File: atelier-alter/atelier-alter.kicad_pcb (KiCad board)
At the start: 2 copper layers, 81.3 x 80 mm, 59 parts, among them SW1 SW_DPST, SW2 SW_DPST, SW3 SW_DPST, SW4 RESET, U1 ATmega32U4-A, U2 PRTR5V0U2X, Y1 16Mhz

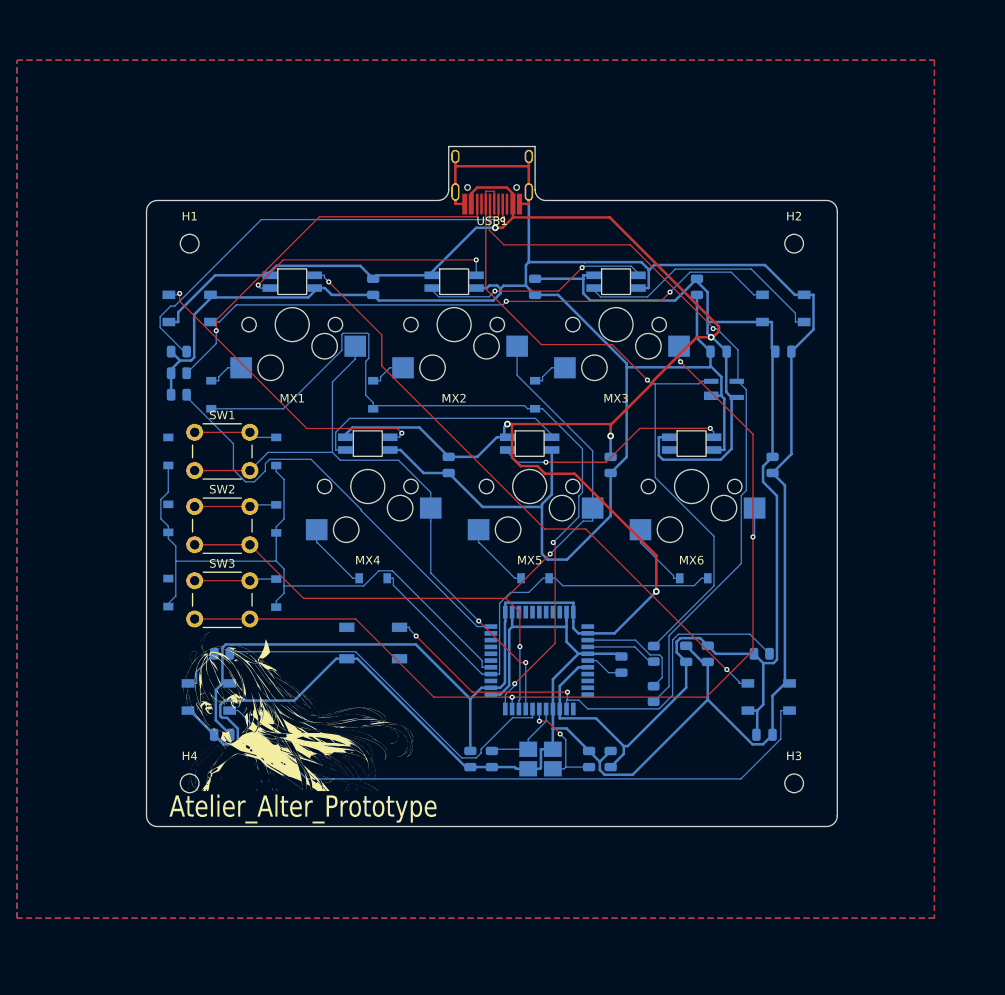
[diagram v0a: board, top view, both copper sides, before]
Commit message: minor updates here and there
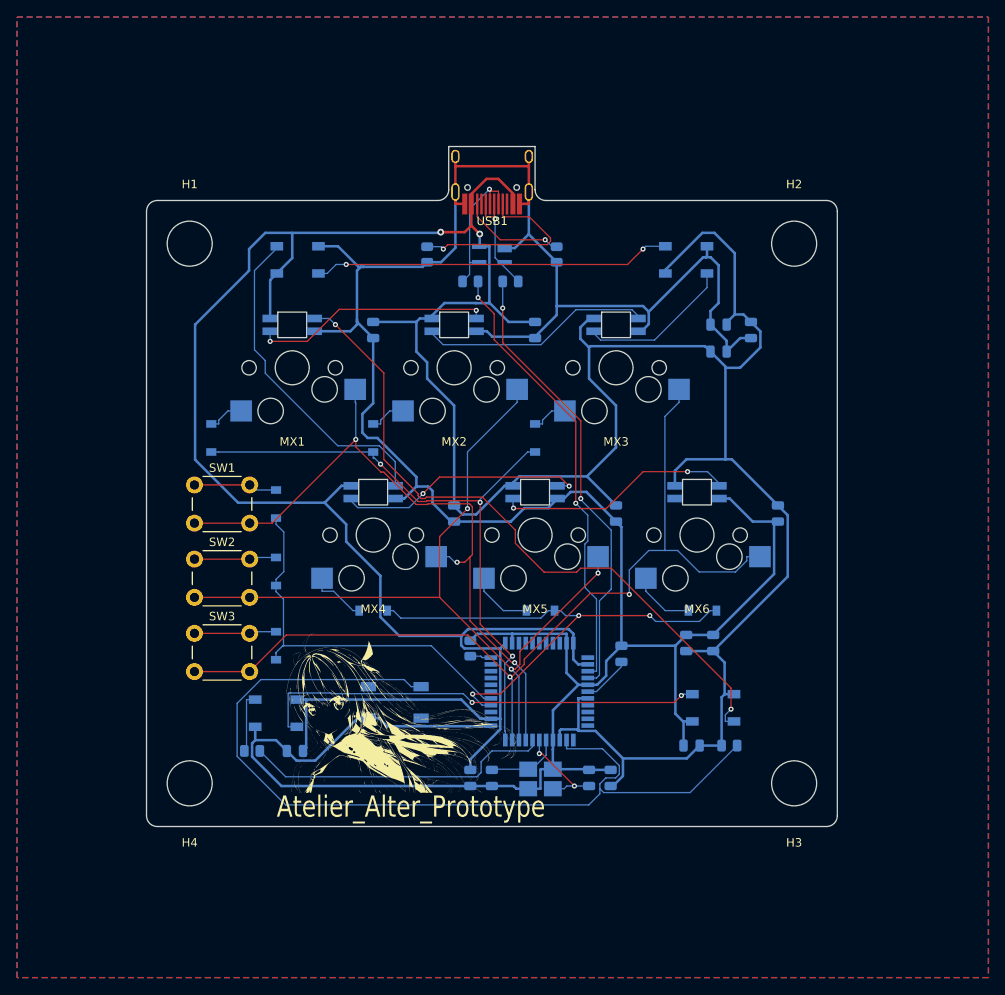
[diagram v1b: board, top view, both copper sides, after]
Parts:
- removed D17, D18, D19: SOD-123, Diode_SMD:D_SOD-123
- H1, H2, H3, H4: footprint MountingHole:MountingHole_2.2mm_M2 -> MountingHole:MountingHole_5.3mm_M5
- moved R1 53.1 mm to (154.9, 70.5), turned to 0 degrees
- moved R2 46.9 mm to (159.7, 70.5), turned to 180 degrees
- moved R5 46.6 mm to (165.1, 67.3), turned to 90 degrees
- moved R6 45.5 mm to (154.9, 113.7), turned to 90 degrees
- moved U2 31.6 mm to (157.5, 67.3), turned to 180 degrees
- moved R4 31.4 mm to (149.9, 67.3), turned to 90 degrees
- moved D14 13.9 mm to (134.6, 67.9)
- moved D9 12.8 mm to (180.3, 67.9)
- moved Atorie' 12.1 mm to (146.7, 120.7)
- moved R7 12.0 mm to (129.3, 125.7)
- moved R3 11.4 mm to (185.4, 125.1)
- moved C10 8.76 mm to (134.3, 125.7)
- moved C11 8.67 mm to (181.0, 125.1), turned to 180 degrees
- moved D2 8.14 mm to (132.1, 121.3)
- moved SW4 7.43 mm to (146.1, 120.0)
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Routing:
- net GND: track 443.9 -> 371.1 mm
- net D-: track 87.2 -> 17.6 mm
- net D+: track 81.9 -> 13.3 mm
- net Net-(R6-Pad1): track 51.8 -> 2.49 mm
- net Net-(R3-Pad1): track 57.7 -> 106.6 mm, vias 2 -> 0
- net Net-(R2-Pad2): track 8.48 -> 53.7 mm, vias 0 -> 2
- net Net-(R1-Pad2): track 13.4 -> 52.9 mm, vias 0 -> 2
- net ROW3: track 78.3 -> 45.2 mm
- net Net-(R5-Pad2): track 44.9 -> 12.3 mm
- net Net-(R4-Pad2): track 52.4 -> 23.6 mm
- net Net-(D14-Pad2): track 68.5 -> 42.1 mm
- net Net-(D2-Pad4): track 74.5 -> 53.4 mm, vias 0 -> 2
- net ROW1: track 93.9 -> 73.7 mm, vias 2 -> 3
- net +5V: track 429.2 -> 442.5 mm, vias 5 -> 2
- net D12: track 29.9 -> 18.1 mm
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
